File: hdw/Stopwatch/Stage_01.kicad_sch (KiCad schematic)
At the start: 5 parts, among them U901 4026, U902 HDSP-7503

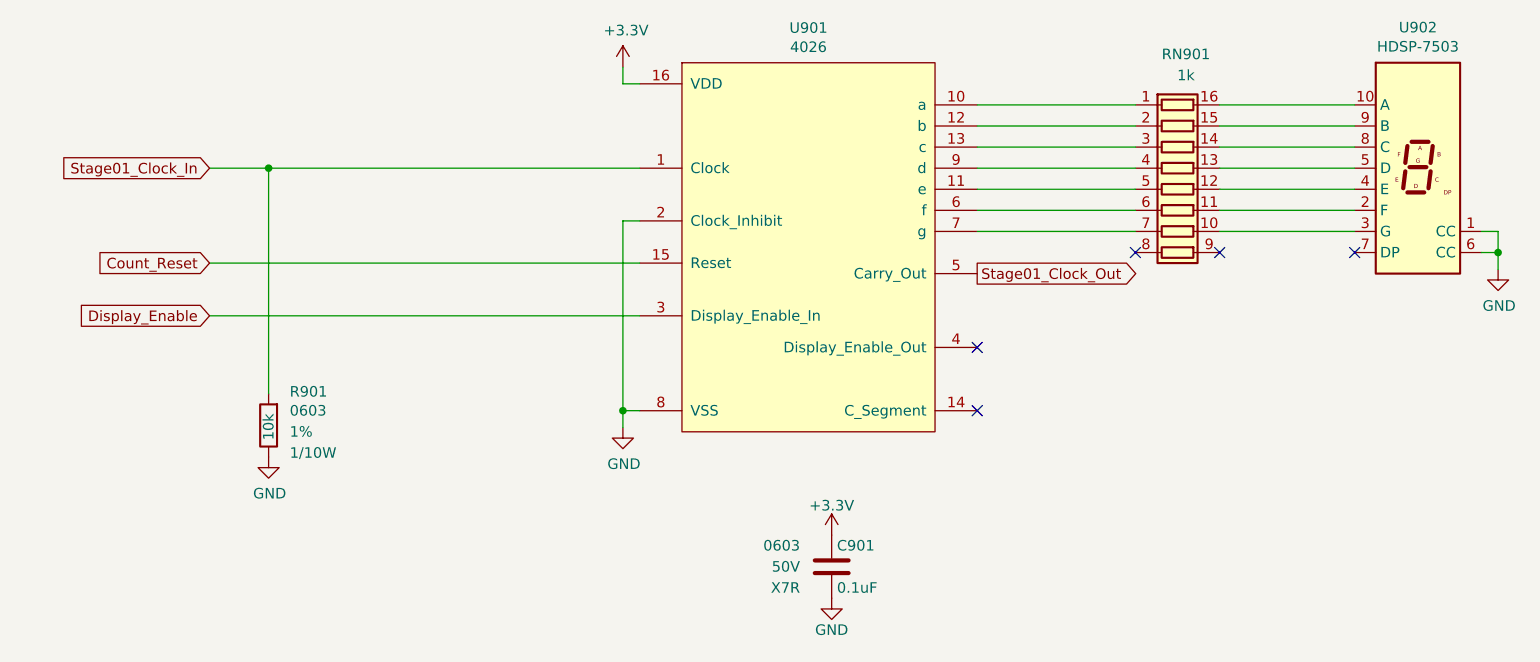
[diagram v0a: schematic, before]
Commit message: started sch work
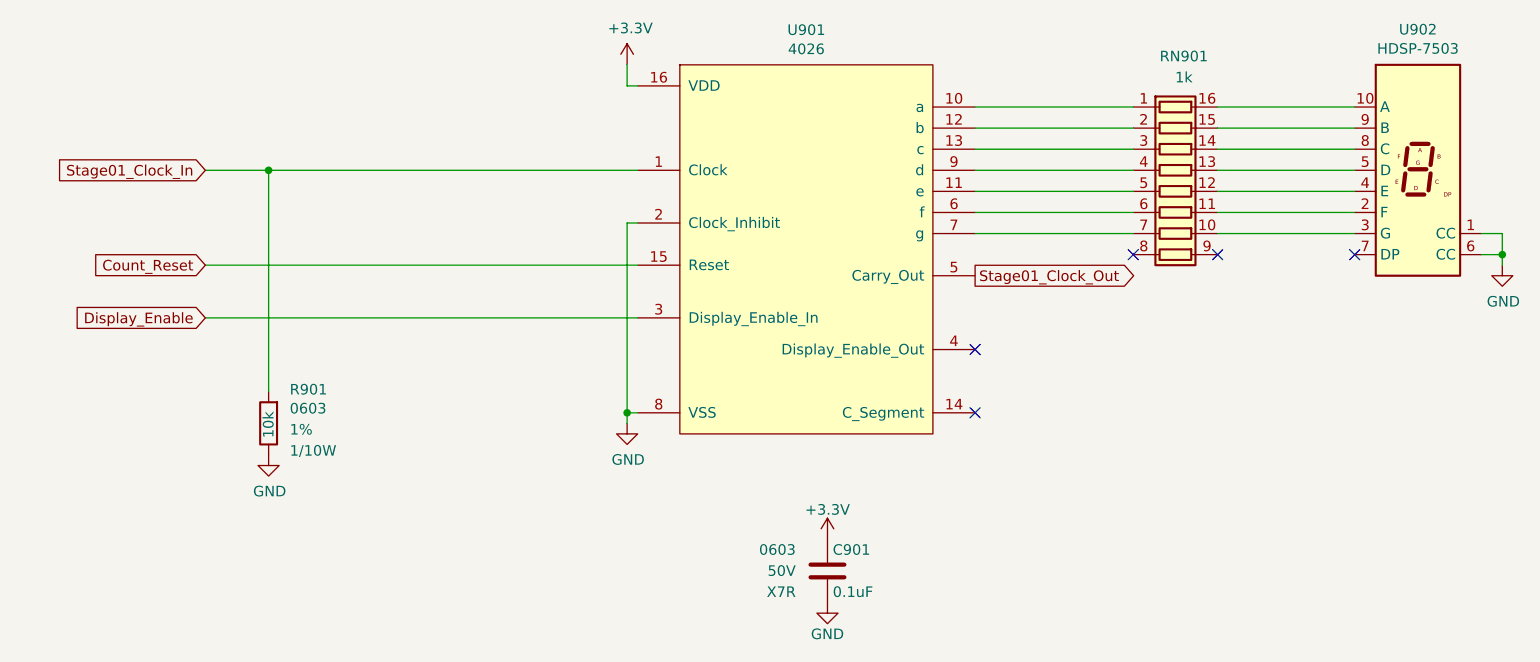
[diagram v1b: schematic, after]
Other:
- moved on the sheet: C901
